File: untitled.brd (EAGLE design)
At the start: 100 x 100 mm, 19 parts, among them X2 pzem-004t

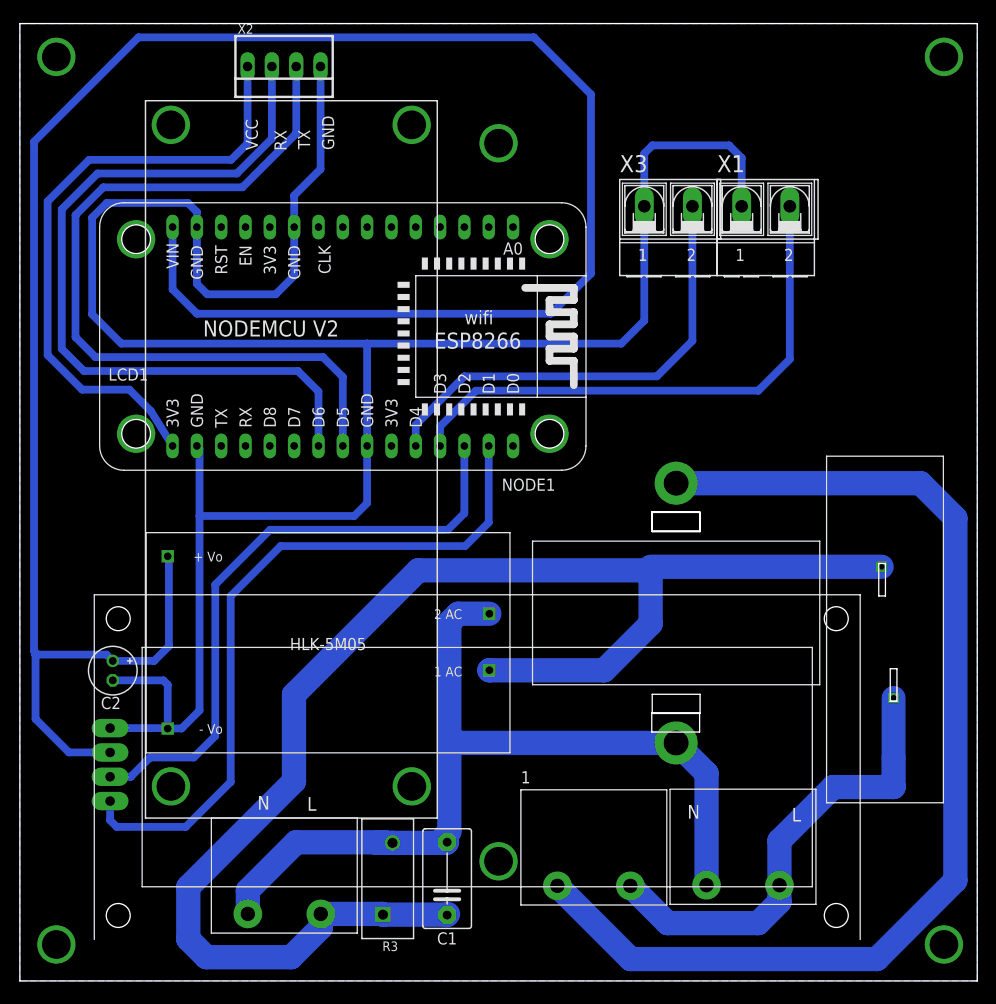
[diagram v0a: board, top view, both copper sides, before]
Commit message: 2158
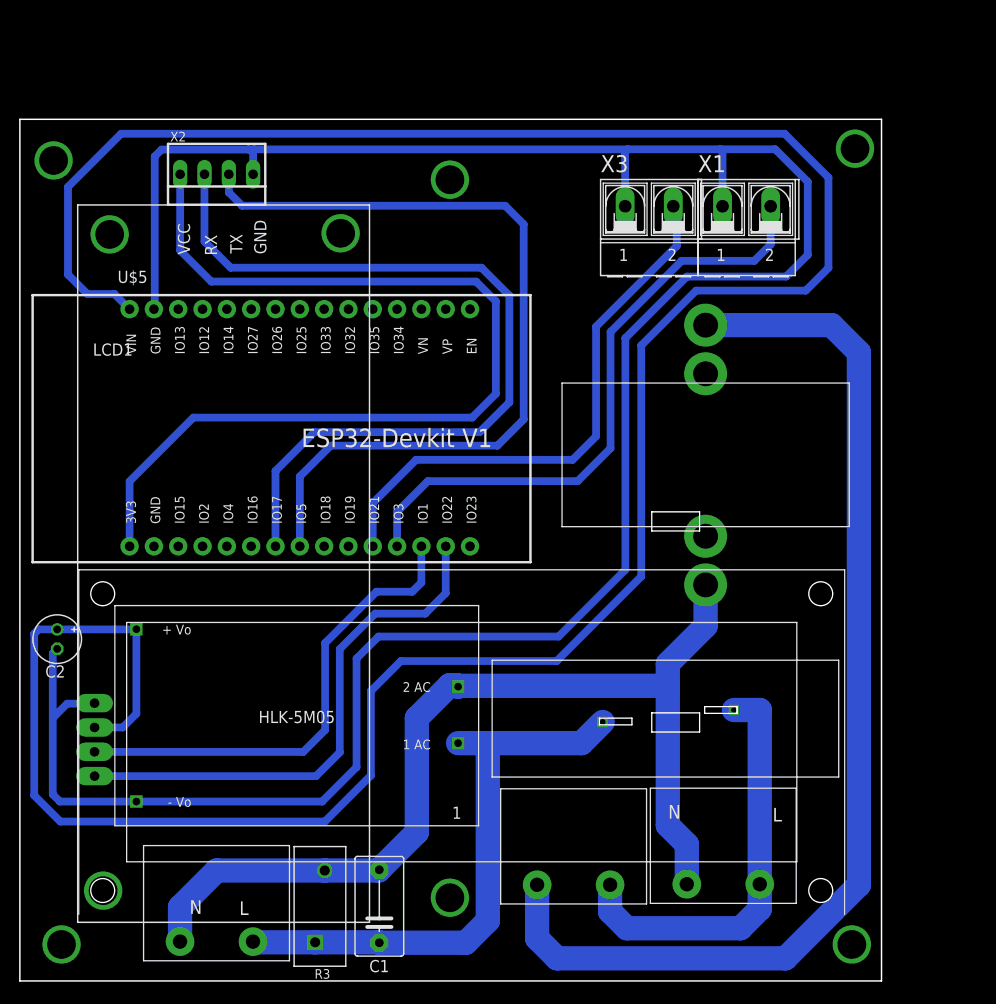
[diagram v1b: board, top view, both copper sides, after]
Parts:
- removed NODE1: NODEMCU_ESP8266, nodemcu_esp8266:NODEMCU_ESP8266
- U$5: value SAPCER -> ESP32DEVKITV1; device spacer:SPACER -> ESP32-DEVKITV1:ESP32-DEVKITV1
- moved U$5 39.2 mm to (34.3, 58.9)
- moved U$8 24.5 mm to (67.7, 27.7), turned to 180 degrees
- moved U$2 16.8 mm to (56.6, 47.5)
- moved U$7 13.5 mm to (33.5, 78.1)
- moved X2 13.3 mm to (20.6, 84.3)
- moved U$3 13.0 mm to (36.5, 81.1)
- moved U$4 13.0 mm to (8.70, 9.43)
- moved U$6 12.8 mm to (3.52, 85.7), turned to 90 degrees
- moved U$1 8.29 mm to (28.9, 27.8)
- moved PZEM 7.65 mm to (12.9, 2.11)
- moved C1 7.65 mm to (37.5, 7.80)
- moved R3 7.65 mm to (31.3, 7.79)
- moved C2 6.68 mm to (3.90, 35.7)
- moved LCD1 3.07 mm to (11.6, 40.4)
- moved 1 2.12 mm to (50.2, 8.04)
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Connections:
- removed net 3V3: NODE1.3V3@2, NODE1.3V3@3
- net 3V: now also U$5.1; no longer NODE1.3V3@1
- net D3: now also U$5.12; no longer NODE1.D3
- net D4: now also U$5.11; no longer NODE1.D4
- net GND: now also U$5.28; no longer NODE1.GND@1, NODE1.GND@2, NODE1.GND@3, NODE1.GND@4
- net RX: now also U$5.7; no longer NODE1.D6
- net SCL: now also U$5.14; no longer NODE1.D1
- net SDA: now also U$5.13; no longer NODE1.D2
- net TX: now also U$5.8; no longer NODE1.D5
- net VCC: now also U$5.30; no longer NODE1.VIN
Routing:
- net N$7: track 152.1 -> 60.1 mm
- net VCC: track 230.9 -> 279.1 mm
- net 3V: track 65.0 -> 101.6 mm
- net SCL: track 74.4 -> 55.8 mm
- net SDA: track 64.7 -> 50.6 mm
- net GND: track 240.7 -> 252.4 mm
- net N$21: track 93.6 -> 105.3 mm
- net D4: track 48.8 -> 58.4 mm
- net D3: track 57.4 -> 65.3 mm
- net RX: track 81.5 -> 87.6 mm
- net N$9: track 48.0 -> 43.5 mm
- net TX: track 83.2 -> 87.6 mm
- net N$2: track 116.7 -> 116.1 mm
- removed copper zone on layer 16, net N$1
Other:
- board size 100 x 100 mm -> 90 x 90 mm
